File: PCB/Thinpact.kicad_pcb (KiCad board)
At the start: 2 copper layers, 228.6 x 116.7 mm, 129 parts, among them SW1 SW_PUSH, SW10 SW_PUSH, SW11 SW_PUSH, SW12 SW_PUSH, SW13 SW_PUSH, SW14 SW_PUSH, SW15 SW_PUSH, SW16 SW_PUSH, SW17 SW_PUSH, SW18 SW_PUSH, SW19 SW_PUSH, SW2 SW_PUSH, SW20 SW_PUSH, SW21 SW_PUSH, SW22 SW_PUSH, SW23 SW_PUSH, SW24 SW_PUSH, SW25 SW_PUSH, SW26 SW_PUSH, SW27 SW_PUSH, SW28 SW_PUSH, SW29 SW_PUSH, SW3 SW_PUSH, SW30 SW_PUSH, SW31 SW_PUSH, SW32 SW_PUSH, SW33 SW_PUSH, SW34 SW_PUSH, SW35 SW_PUSH, SW36 SW_PUSH, SW37 SW_PUSH, SW38 SW_PUSH, SW39 SW_PUSH, SW4 SW_PUSH, SW40 SW_PUSH, SW41 SW_PUSH, SW42 SW_PUSH, SW43 SW_PUSH, SW44 SW_PUSH, SW45 SW_PUSH, SW46 SW_PUSH, SW47 SW_PUSH, SW48 SW_PUSH, SW49 SW_PUSH, SW5 SW_PUSH, SW50 SW_PUSH, SW51 SW_PUSH, SW52 SW_PUSH, SW53 SW_PUSH, SW54 SW_PUSH, SW55 SW_PUSH, SW56 SW_PUSH, SW57 SW_PUSH, SW58 SW_PUSH, SW59 SW_PUSH, SW6 SW_PUSH, SW60 SW_SPDT, SW61 SW_SPDT, SW7 SW_PUSH, SW8 SW_PUSH, SW9 SW_PUSH, U1 Micon_BLEMicroPro, U2 Micon_BLEMicroPro

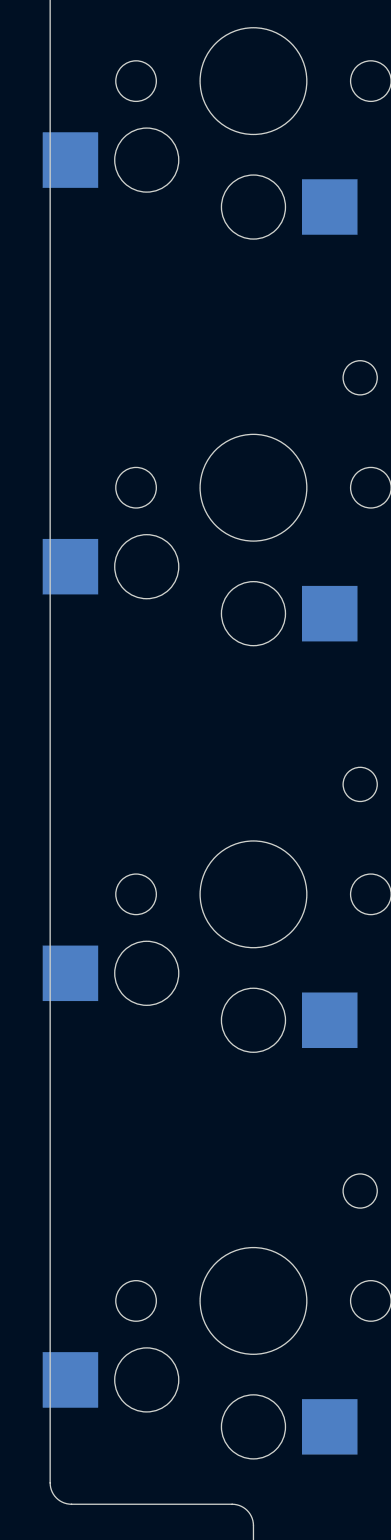
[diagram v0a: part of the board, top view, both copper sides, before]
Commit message: Update sch and kicad_pcb
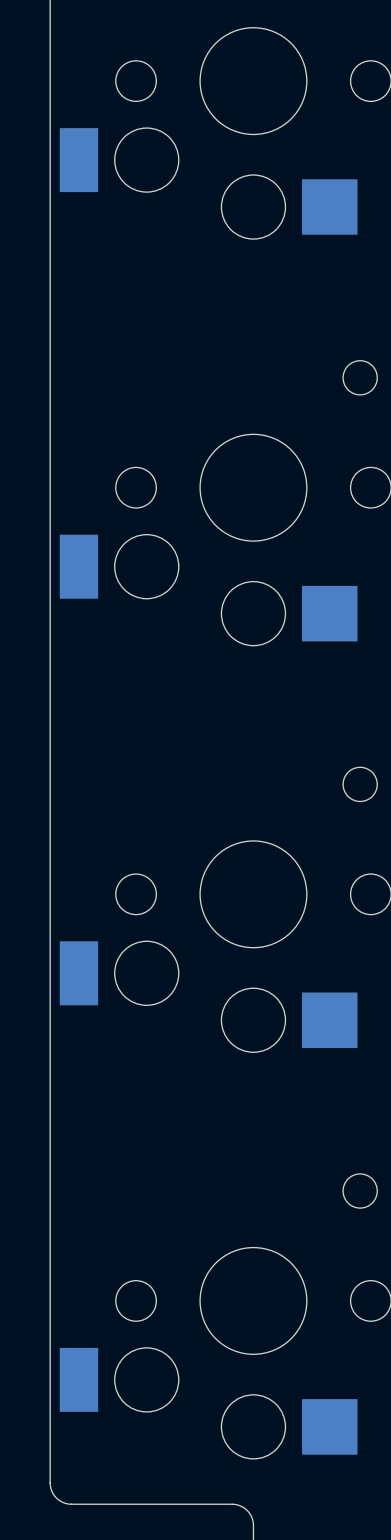
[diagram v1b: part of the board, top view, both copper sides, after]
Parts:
- SW1, SW2, SW3, SW4: footprint footprints:Choc_Hotswap_1u -> footprints:Choc_Hotswap_1u_Small
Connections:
- U1 pad 21: VCC -> unconnected-(U1-VCC-Pad21)
- U2 pad 21: VCC -> unconnected-(U2-VCC-Pad21)
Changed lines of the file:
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@@
 	(net 5 "col5")
 	(net 6 "row3")
-	(net 7 "VCC")
+	(net 7 "unconnected-(U2-VCC-Pad21)")
 	(net 8 "row9")
 	(net 9 "col0")
@@
 	(net 89 "unconnected-(SW60-C-Pad3)")
 	(net 90 "Net-(D61-A)")
+	(net 91 "unconnected-(U1-VCC-Pad21)")
 	(footprint "footprints:Choc_Hotswap_1u"
 		(layer "F.Cu")
@@
 			(layers "*.Cu" "*.Mask" "F.SilkS")
 			(remove_unused_layers no)
-			(net 7 "VCC")
+			(net 7 "unconnected-(U2-VCC-Pad21)")
 			(pinfunction "VCC")
-			(pintype "power_in")
+			(pintype "power_in+no_connect")
 		)
 		(pad "22" thru_hole circle
@@
 		(embedded_fonts no)
 	)
-	(footprint "footprints:Choc_Hotswap_1u"
+	(footprint "footprints:Choc_Hotswap_1u_Small"
 		(layer "F.Cu")
 		(at 38.1 90.4875)
-		(descr "Supported: Choc v1/v2, hotswap, 1u")
+		(descr "Supported: Choc v1/v2, hotswap, 1u. This is for edge-located key switches.")
 		(property "Reference" "SW2"
 			(at -5.08 -6.35 180)
@@
 		)
 		(pad "1" smd rect
-			(at -8.575 3.7 180)
-			(size 2.6 2.6)
+			(at -8.175 3.7 180)
+			(size 1.8 3)
 			(layers "B.Cu" "B.Mask" "B.Paste")
 			(net 9 "col0")
@@
 		)
 	)
-	(footprint "footprints:Choc_Hotswap_1u"
+	(footprint "footprints:Choc_Hotswap_1u_Small"
 		(layer "F.Cu")
 		(at 38.1 109.5375)
-		(descr "Supported: Choc v1/v2, hotswap, 1u")
+		(descr "Supported: Choc v1/v2, hotswap, 1u. This is for edge-located key switches.")
 		(property "Reference" "SW3"
 			(at -5.08 -6.35 180)
@@
 		)
 		(pad "1" smd rect
-			(at -8.575 3.7 180)
-			(size 2.6 2.6)
+			(at -8.175 3.7 180)
+			(size 1.8 3)
 			(layers "B.Cu" "B.Mask" "B.Paste")
 			(net 9 "col0")
@@
 		(embedded_fonts no)
 	)
-	(footprint "footprints:Choc_Hotswap_1u"
+	(footprint "footprints:Choc_Hotswap_1u_Small"
 		(layer "F.Cu")
 		(at 38.1 71.4375)
-		(descr "Supported: Choc v1/v2, hotswap, 1u")
+		(descr "Supported: Choc v1/v2, hotswap, 1u. This is for edge-located key switches.")
 		(property "Reference" "SW1"
 			(at -5.08 -6.35 180)
@@
 		)
 		(pad "1" smd rect
-			(at -8.575 3.7 180)
-			(size 2.6 2.6)
+			(at -8.175 3.7 180)
+			(size 1.8 3)
 			(layers "B.Cu" "B.Mask" "B.Paste")
 			(net 9 "col0")
@@
 			(layers "*.Cu" "*.Mask" "F.SilkS")
 			(remove_unused_layers no)
-			(net 7 "VCC")
+			(net 91 "unconnected-(U1-VCC-Pad21)")
 			(pinfunction "VCC")
-			(pintype "power_in")
+			(pintype "power_in+no_connect")
 		)
 		(pad "22" thru_hole circle
@@
 		)
 	)
-	(footprint "footprints:Choc_Hotswap_1u"
+	(footprint "footprints:Choc_Hotswap_1u_Small"
 		(layer "F.Cu")
 		(at 38.1 128.5875)
-		(descr "Supported: Choc v1/v2, hotswap, 1u")
+		(descr "Supported: Choc v1/v2, hotswap, 1u. This is for edge-located key switches.")
 		(property "Reference" "SW4"
 			(at -5.08 -6.35 180)
@@
 		)
 		(pad "1" smd rect
-			(at -8.575 3.7 180)
-			(size 2.6 2.6)
+			(at -8.175 3.7 180)
+			(size 1.8 3)
 			(layers "B.Cu" "B.Mask" "B.Paste")
 			(net 9 "col0")
